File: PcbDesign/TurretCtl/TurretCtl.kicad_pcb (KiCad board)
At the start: 4 copper layers, 70.4 x 53.8 mm, 67 parts, among them J1 FLIR, J2 Stepper1, J3 Stepper2, J4 PWR, J5 Sensors

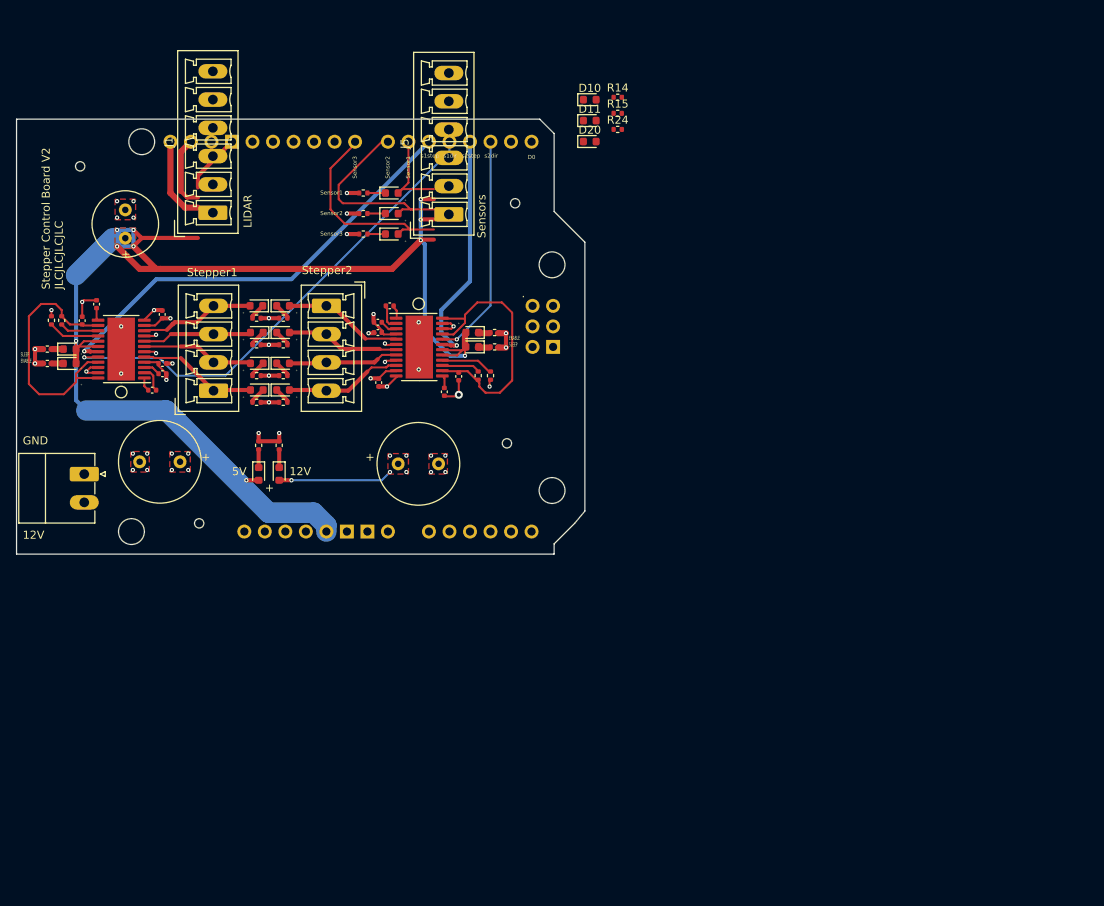
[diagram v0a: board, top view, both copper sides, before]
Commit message: New Layout
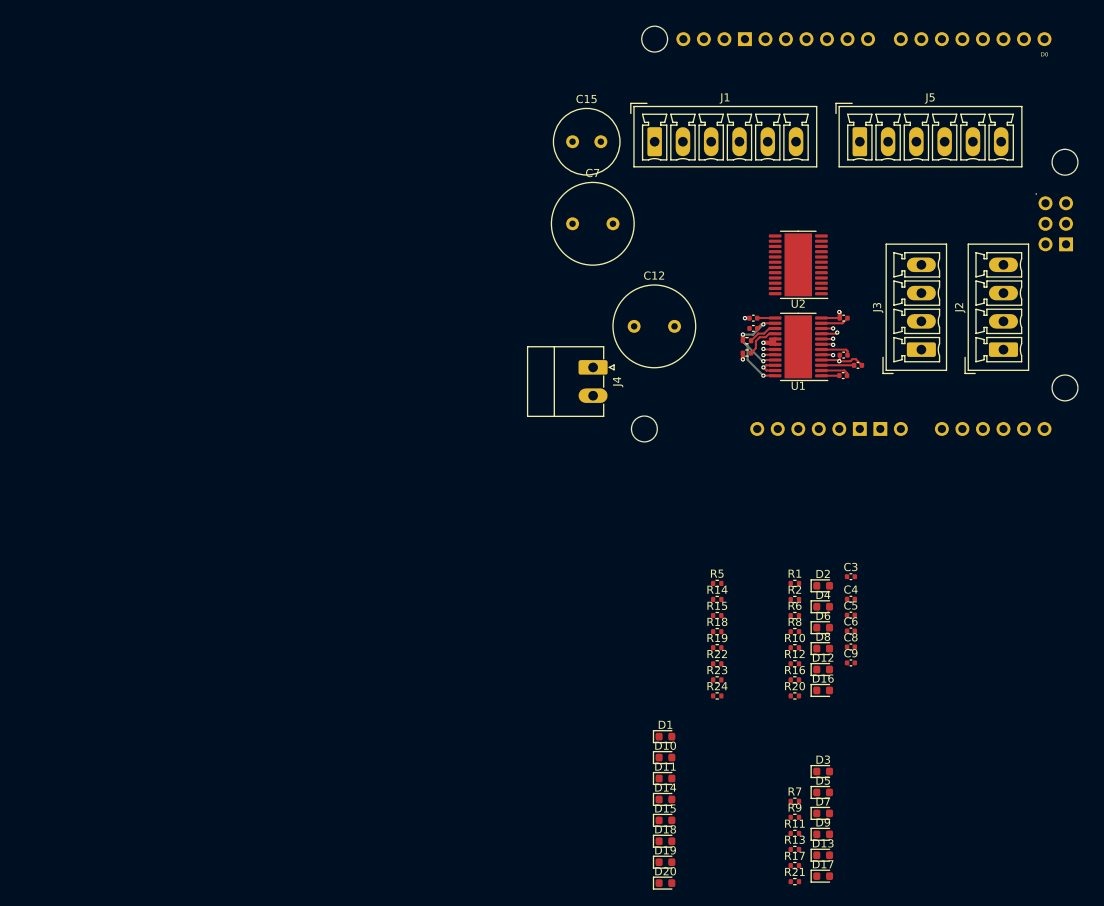
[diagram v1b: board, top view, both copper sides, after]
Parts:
- moved C9 103.4 mm to (125.9, 128.0), turned to 0 degrees
- moved C8 103.4 mm to (125.9, 126.0), turned to 0 degrees
- moved D16 101.7 mm to (122.5, 131.4)
- moved D12 101.4 mm to (122.5, 128.8)
- moved R20 101.3 mm to (119.0, 132.1), turned to 0 degrees
- moved R16 101.2 mm to (119.0, 130.1), turned to 0 degrees
- moved J2 97.9 mm to (144.8, 89.2)
- moved R1 97.6 mm to (119.0, 118.2), turned to 0 degrees
- moved R2 97.1 mm to (119.0, 120.2), turned to 0 degrees
- moved D9 93.5 mm to (122.5, 149.2)
- moved C5 93.0 mm to (125.9, 122.1), turned to 0 degrees
- moved D20 92.3 mm to (102.9, 155.3)
- moved C6 91.4 mm to (125.9, 124.1)
- moved R13 91.3 mm to (119.0, 151.1), turned to 0 degrees
- moved C4 89.7 mm to (125.9, 120.1), turned to 0 degrees
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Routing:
- net +5V: track 176.6 -> 3.18 mm, vias 10 -> 1
- net S1_DIR: track 60.6 -> 0.00 mm, vias 1 -> 0
- net S1_STEP: track 56.0 -> 0.00 mm, vias 1 -> 0
- net GND: track 61.6 -> 13.4 mm, vias 43 -> 5
- net /Stepper1/DVDD: track 33.2 -> 0.00 mm
- net S2_STEP: track 30.4 -> 1.48 mm
- net S2_DIR: track 28.0 -> 1.47 mm
- net D8: track 25.2 -> 0.00 mm
- net D7: track 24.4 -> 0.00 mm
- net +12V: track 30.2 -> 9.79 mm, vias 13 -> 1
- net S1_AOUT2: track 15.5 -> 0.00 mm
- net S1_AOUT1: track 14.9 -> 0.00 mm
- net S1_BOUT1: track 14.4 -> 0.00 mm
- net S2_AOUT2: track 15.6 -> 1.48 mm, vias 0 -> 1
- net /Stepper2/DVDD: track 33.0 -> 19.0 mm, vias 0 -> 4
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- removed copper zone on F.Cu, net +12V
- removed copper zone on B.Cu, net +5V
- removed copper zone on F.Cu, net +5V
- removed copper zone on F.Cu, net GND
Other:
- board outline removed
- board text removed: "+"
- board text removed: "12V"
- board text removed: "5V"
- board text removed: "ENABLE SLEEP"
- board text removed: "GND"
- board text removed: "LIDAR"
- board text removed: "SLEEP ENABLE"
- board text removed: "Sensor1"
- board text removed: "Sensor2"
- board text removed: "Sensor3"
- board text removed: "Sensors"
- board text removed: "Stepper Control Board V2 JLCJLCJLCJLC"
- board text removed: "Stepper1"
- board text removed: "Stepper2"
- board text removed: "s1dir"
- board text removed: "s1step"
- board text removed: "s2dir"
- board text removed: "s2step"

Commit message: Control board v3
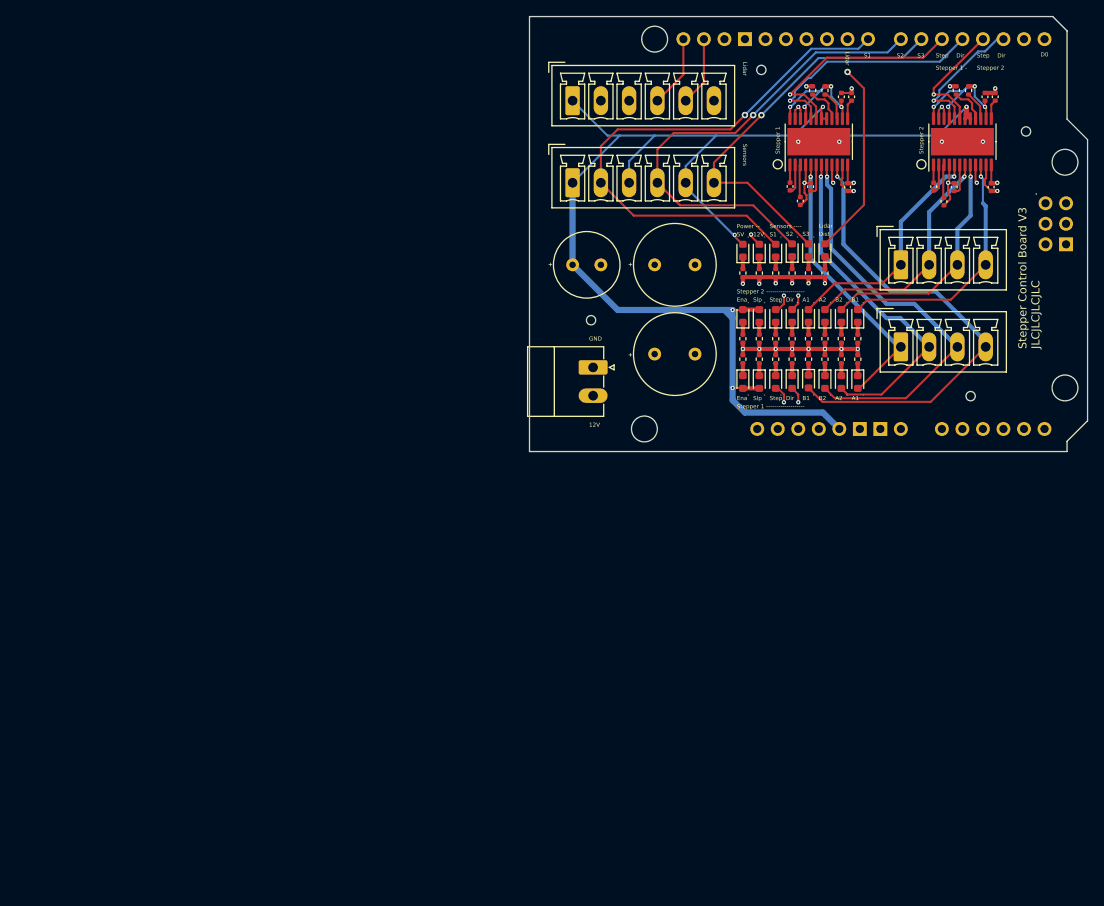
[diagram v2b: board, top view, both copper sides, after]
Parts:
- added D21: LED, LED_SMD:LED_0603_1608Metric, F.Cu at (116.6, 93.2)
- added D22: LED, LED_SMD:LED_0603_1608Metric, F.Cu at (118.6, 93.2)
- added R25: 330, Resistor_SMD:R_0402_1005Metric, F.Cu at (116.6, 90.4)
- added R26: 330, Resistor_SMD:R_0402_1005Metric, F.Cu at (118.6, 90.4)
- moved D19 76.9 mm to (116.6, 77.0), turned to 90 degrees
- moved D18 74.8 mm to (118.6, 76.9), turned to 90 degrees
- moved D15 72.8 mm to (120.7, 76.9), turned to 90 degrees
- moved D20 71.9 mm to (118.6, 85.1), turned to 90 degrees
- moved C9 70.1 mm to (126.0, 57.9), turned to 90 degrees
- moved D17 70.1 mm to (112.5, 85.1), turned to 90 degrees
- moved D14 68.6 mm to (112.5, 77.0), turned to 90 degrees
- moved C8 68.1 mm to (124.7, 57.9), turned to 90 degrees
- moved R21 67.5 mm to (112.5, 87.9), turned to -90 degrees
- moved D13 67.2 mm to (114.6, 85.1), turned to 90 degrees
- moved D10 65.8 mm to (122.7, 76.9), turned to 90 degrees
- moved R17 65.4 mm to (114.6, 87.9), turned to -90 degrees
- moved D9 64.2 mm to (120.7, 85.1), turned to 90 degrees
- moved R13 63.3 mm to (120.7, 87.9), turned to -90 degrees
- moved R2 63.1 mm to (122.7, 57.2), turned to -90 degrees
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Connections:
- D10 pad 2: GND -> Net-(D10-A)
- D11 pad 2: SDA -> S2_STEP
- D20 pad 2: SCL -> S2_DIR
- XA1 pad D9: unconnected-(XA1-PadD9) -> Net-(D10-A)
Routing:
- net +5V: track 3.18 -> 162.2 mm, vias 1 -> 5
- net S1_DIR: track 0.00 -> 71.5 mm, vias 0 -> 2
- net S1_STEP: track 0.00 -> 69.6 mm, vias 0 -> 2
- net D8: track 0.00 -> 67.9 mm, vias 0 -> 1
- net D7: track 0.00 -> 59.9 mm, vias 0 -> 1
- net S1_BOUT1: track 0.00 -> 58.9 mm, vias 0 -> 1
- net GND: track 13.4 -> 71.4 mm, vias 5 -> 28
- net S2_STEP: track 1.48 -> 52.6 mm, vias 1 -> 2
- net S2_DIR: track 1.47 -> 52.4 mm, vias 1 -> 2
- net S1_BOUT2: track 0.00 -> 50.8 mm, vias 0 -> 1
- net D6: track 0.00 -> 49.3 mm, vias 0 -> 1
- net S1_AOUT2: track 0.00 -> 42.7 mm, vias 0 -> 1
- net S1_AOUT1: track 0.00 -> 34.8 mm, vias 0 -> 1
- net S2_BOUT1: track 1.46 -> 30.8 mm
- net S2_BOUT2: track 1.47 -> 29.7 mm
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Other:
- board outline added: 69.1 x 53.8 mm
- board text added: "+"
- board text added: "12V"
- board text added: "5V"
- board text added: "A1"
- board text added: "A2"
- board text added: "B1"
- board text added: "B2"
- board text added: "Dir"
- board text added: "Dist"
- board text added: "Ena"
- board text added: "GND"
- board text added: "Lidar"
- board text added: "Power --"
- board text added: "S1"
- board text added: "S2"
- board text added: "S3"
- board text added: "Sensors"
- board text added: "Sensors ----"
- board text added: "Slp"
- board text added: "Step"
- board text added: "Stepper 1"
- board text added: "Stepper 1 -"
- board text added: "Stepper 1 -------------------"
- board text added: "Stepper 2"
- board text added: "Stepper 2 -------------------"
- board text added: "Stepper Control Board V3 JLCJLCJLCJLC"
